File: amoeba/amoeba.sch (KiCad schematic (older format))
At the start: 10 parts

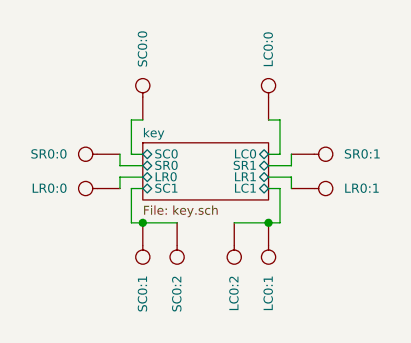
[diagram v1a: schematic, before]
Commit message: Update amoeba to v1.2.1
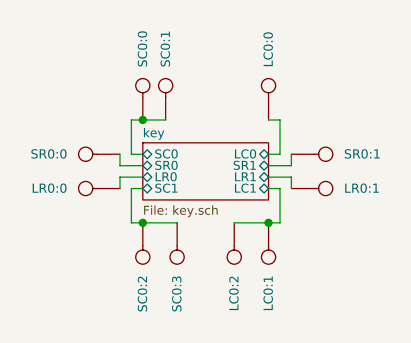
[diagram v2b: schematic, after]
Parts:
- added SC0:1: CONN_1, symbol CONN_1
- renumbered SC0:1 to SC0:2, SC0:2 to SC0:3
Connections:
- net key/SC0: now also SC0:1.1
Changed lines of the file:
@@
 Sheet 1 4
 Title ""
-Date "25 aug 2015"
+Date "13 sep 2015"
 Rev ""
 Comp ""
@@
 $EndComp
 $Comp
-L CONN_1 SC0:1
+L CONN_1 SC0:2
 U 1 1 55D71CCC
 P 4300 3450
-F 0 "SC0:1" H 4380 3450 40  0000 L CNN
+F 0 "SC0:2" H 4380 3450 40  0000 L CNN
 F 1 "CONN_1" H 4300 3505 30  0001 C CNN
 F 2 "" H 4300 3450 60  0000 C CNN
@@
 	4250 3000 4250 2850
 Wire Wire Line
-	4250 2850 4300 2850
+	4250 2850 4400 2850
 Wire Wire Line
 	4850 3000 4900 3000
@@
 $EndSheet
 $Comp
-L CONN_1 SC0:2
+L CONN_1 SC0:3
 U 1 1 55D928B8
 P 4450 3450
-F 0 "SC0:2" H 4530 3450 40  0000 L CNN
+F 0 "SC0:3" H 4530 3450 40  0000 L CNN
 F 1 "CONN_1" H 4450 3505 30  0001 C CNN
 F 2 "" H 4450 3450 60  0000 C CNN
@@
 Connection ~ 4850 3300
 Connection ~ 4300 3300
+$Comp
+L CONN_1 SC0:1
+U 1 1 55F593C9
+P 4400 2700
+F 0 "SC0:1" H 4480 2700 40  0000 L CNN
+F 1 "CONN_1" H 4400 2755 30  0001 C CNN
+F 2 "" H 4400 2700 60  0000 C CNN
+F 3 "" H 4400 2700 60  0000 C CNN
+	1    4400 2700
+	0    -1   -1   0
+$EndComp
+Connection ~ 4300 2850
 $EndSCHEMATC
